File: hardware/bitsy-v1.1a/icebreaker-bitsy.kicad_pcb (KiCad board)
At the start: 4 copper layers, 35.6 x 17.8 mm, 99 parts, among them J1 USB_C, P0 0, P1 1, P10 10, P11 11, P12 12, P13 13, P14 14, P15 15, P16 16, P17 17, P18 18, P19 19, P2 2, P20 20, P21 21, P22 22, P23 23, P24 GND, P25 GND, P26 GND, P27 3V3, P28 3V3, P29 VIN, P3 3, P30 CDONE, P31 CRESET, P32 UP, P33 UP, P34 UP, P35 UP, P36 CS, P37 SCK, P38 MISO, P39 MOSI, P4 4, P40 IO3, P41 IO2, P5 5, P6 6, P7 7, P8 8, P9 9, SW1 TACT, U1 USBLC6-2, U2 TLV75533PDRV, U3 TLV75512PDRV, U4 LY68L6400, U5 W25Q, U6 ICE40UP5K-SG48, X1 12MHz

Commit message: More WIP
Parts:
- turned SW1 to 0 degrees
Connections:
- SW1 pad 1: /~BTN -> GND
- SW1 pad 2: GND -> /~BTN

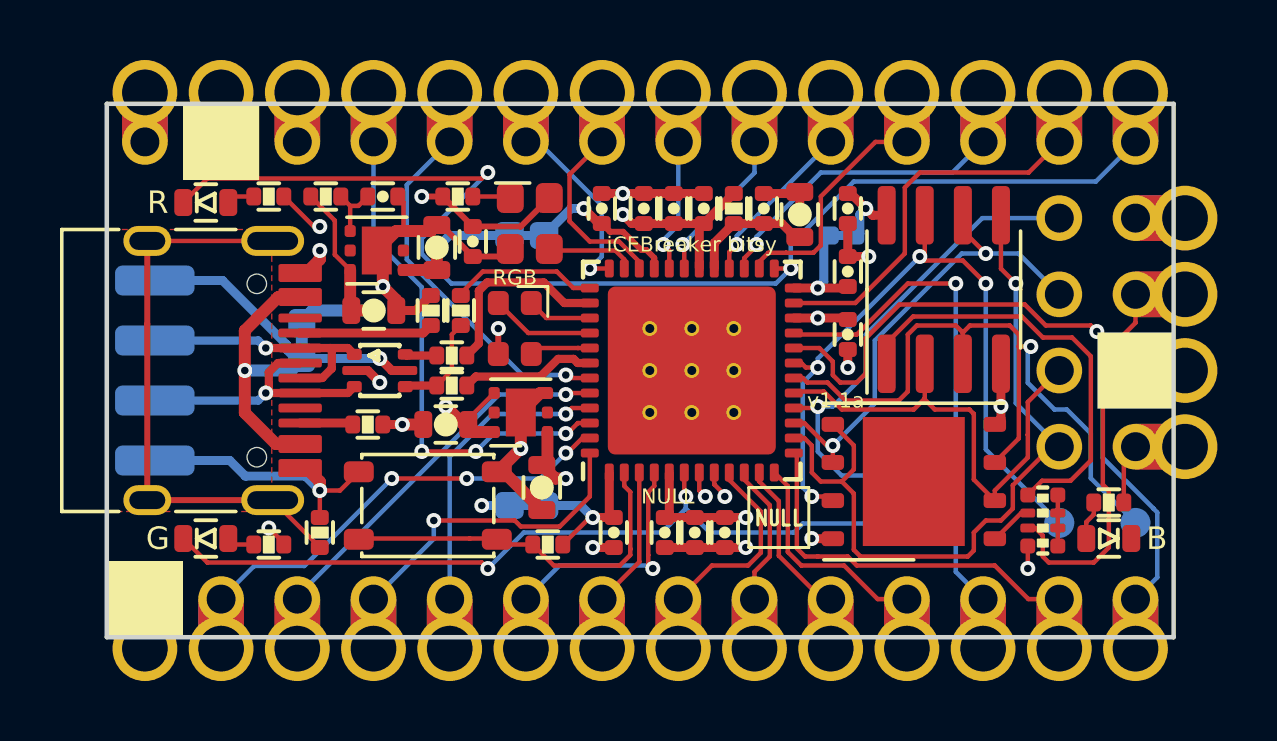
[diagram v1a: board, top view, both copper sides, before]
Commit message: More routing
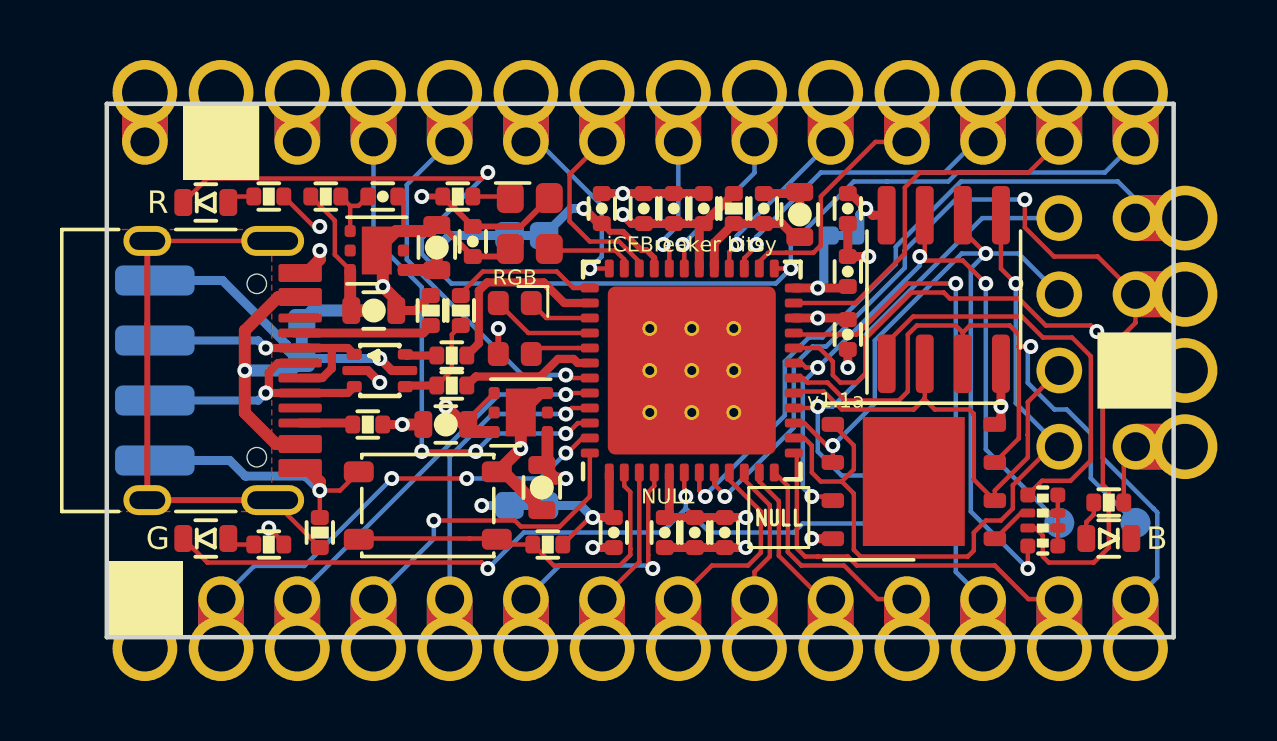
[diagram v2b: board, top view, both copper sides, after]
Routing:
- net /CDONE: track 2.19 -> 23.4 mm
- net /~CRESET: track 13.7 -> 34.9 mm, vias 1 -> 2
- net /SPI_SCK: track 16.5 -> 28.0 mm
- net /RAM_~CS: track 14.5 -> 15.7 mm
